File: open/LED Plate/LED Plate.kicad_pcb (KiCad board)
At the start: 2 copper layers, 10 x 13.5 mm, 2 parts, among them J1 Conn_01x02

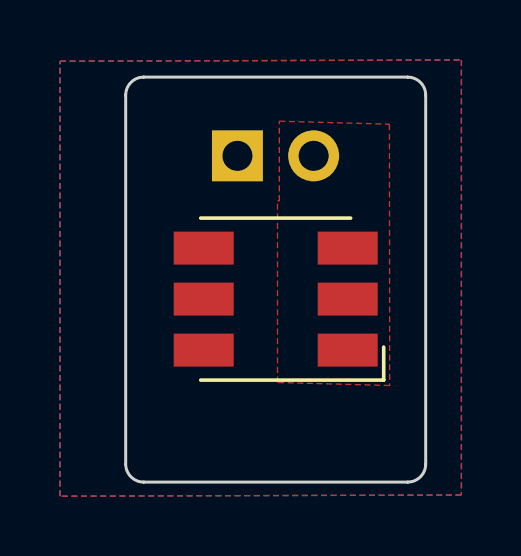
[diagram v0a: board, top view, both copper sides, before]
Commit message: L1-Final Version, L1 Single MUX test
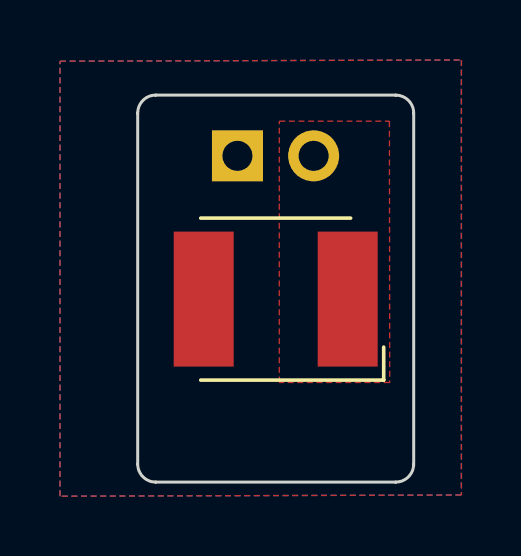
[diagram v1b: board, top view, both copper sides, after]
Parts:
- D1: value LED_RGB -> LED; footprint LED_SMD:LED_RGB_5050-6 -> 2024l1:LED5050
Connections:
- D1 pad 1: +3V3 -> GND
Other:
- board size 10 x 13.5 mm -> 9.2 x 12.9 mm
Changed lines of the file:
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@@
   (net 1 "GND")
   (net 2 "+3V3")
-  (footprint "LED_SMD:LED_RGB_5050-6" (layer "F.Cu")
+  (footprint "2024l1:LED5050" (layer "F.Cu")
     (at 148.5 105.4 180)
-    (descr "http://cdn.sparkfun.com/datasheets/Components/LED/5060BRG4.pdf")
-    (tags "RGB LED 5050-6")
     (property "Sheetfile" "LED Plate.kicad_sch")
     (property "Sheetname" "")
-    (property "ki_description" "RGB LED, 6 pin package")
-    (property "ki_keywords" "LED RGB diode")
+    (property "ki_description" "Light emitting diode")
+    (property "ki_keywords" "LED diode")
     (attr smd)
-    (fp_text reference "D1" (at 0 -3.5) (layer "F.SilkS") hide
-        (effects (font (size 1 1) (thickness 0.15)))
-    )
-    (fp_text value "LED_RGB" (at 0 3.3) (layer "F.Fab")
+    (fp_text reference "D1" (at 0 -0.5 180 unlocked) (layer "F.SilkS") hide
+        (effects (font (size 1 1) (thickness 0.1)))
+    )
+    (fp_text value "LED" (at 0 1 180 unlocked) (layer "F.Fab")
         (effects (font (size 1 1) (thickness 0.15)))
     )
@@
     (fp_circle (center 0 0) (end 0 -1.9)
       (stroke (width 0.1) (type solid)) (fill none) (layer "F.Fab"))
-    (pad "1" smd rect (at -2.4 -1.7 270) (size 1.1 2) (layers "F.Cu" "F.Paste" "F.Mask")
-      (net 2 "+3V3") (pinfunction "RK") (pintype "passive"))
-    (pad "2" smd rect (at -2.4 0 270) (size 1.1 2) (layers "F.Cu" "F.Paste" "F.Mask")
-      (net 2 "+3V3") (pinfunction "GK") (pintype "passive"))
-    (pad "3" smd rect (at -2.4 1.7 270) (size 1.1 2) (layers "F.Cu" "F.Paste" "F.Mask")
-      (net 2 "+3V3") (pinfunction "BK") (pintype "passive"))
-    (pad "4" smd rect (at 2.4 1.7 270) (size 1.1 2) (layers "F.Cu" "F.Paste" "F.Mask")
-      (net 1 "GND") (pinfunction "BA") (pintype "passive"))
-    (pad "5" smd rect (at 2.4 0 270) (size 1.1 2) (layers "F.Cu" "F.Paste" "F.Mask")
-      (net 1 "GND") (pinfunction "GA") (pintype "passive"))
-    (pad "6" smd rect (at 2.4 -1.7 270) (size 1.1 2) (layers "F.Cu" "F.Paste" "F.Mask")
-      (net 1 "GND") (pinfunction "RA") (pintype "passive"))
-    (model "${KICAD6_3DMODEL_DIR}/LED_SMD.3dshapes/LED_RGB_5050-6.wrl"
-      (offset (xyz 0 0 0))
-      (scale (xyz 1 1 1))
-      (rotate (xyz 0 0 0))
-    )
+    (pad "1" smd rect (at 2.4 0 270) (size 4.5 2) (layers "F.Cu" "F.Paste" "F.Mask")
+      (net 1 "GND") (pinfunction "K") (pintype "passive"))
+    (pad "2" smd rect (at -2.4 0 270) (size 4.5 2) (layers "F.Cu" "F.Paste" "F.Mask")
+      (net 2 "+3V3") (pinfunction "A") (pintype "passive"))
   )
   (footprint "Connector_PinHeader_2.54mm:PinHeader_1x02_P2.54mm_Horizontal" (layer "B.Cu")
@@
     )
   )
-  (gr_line (start 144.1 111.5) (end 152.9 111.5)
-    (stroke (width 0.1) (type default)) (layer "Edge.Cuts"))
-  (gr_line (start 143.5 98.6) (end 143.5 110.9)
-    (stroke (width 0.1) (type default)) (layer "Edge.Cuts"))
-  (gr_line (start 153.5 98.6) (end 153.5 110.9)
-    (stroke (width 0.1) (type default)) (layer "Edge.Cuts"))
-  (gr_arc (start 152.9 98) (mid 153.324264 98.175736) (end 153.5 98.6)
-    (stroke (width 0.1) (type default)) (layer "Edge.Cuts"))
-  (gr_arc (start 144.1 111.5) (mid 143.675736 111.324264) (end 143.5 110.9)
-    (stroke (width 0.1) (type default)) (layer "Edge.Cuts"))
-  (gr_arc (start 153.5 110.9) (mid 153.324264 111.324264) (end 152.9 111.5)
-    (stroke (width 0.1) (type default)) (layer "Edge.Cuts"))
-  (gr_arc (start 143.5 98.6) (mid 143.675736 98.175736) (end 144.1 98)
-    (stroke (width 0.1) (type default)) (layer "Edge.Cuts"))
-  (gr_line (start 144.1 98) (end 152.9 98)
-    (stroke (width 0.1) (type default)) (layer "Edge.Cuts"))
+  (gr_line (start 144.5 111.5) (end 152.5 111.5)
+    (stroke (width 0.1) (type default)) (layer "Edge.Cuts"))
+  (gr_arc (start 152.5 98.6) (mid 152.924264 98.775736) (end 153.1 99.2)
+    (stroke (width 0.1) (type default)) (layer "Edge.Cuts"))
+  (gr_arc (start 144.5 111.5) (mid 144.075736 111.324264) (end 143.9 110.9)
+    (stroke (width 0.1) (type default)) (layer "Edge.Cuts"))
+  (gr_arc (start 153.1 110.9) (mid 152.924264 111.324264) (end 152.5 111.5)
+    (stroke (width 0.1) (type default)) (layer "Edge.Cuts"))
+  (gr_line (start 143.9 99.2) (end 143.9 110.9)
+    (stroke (width 0.1) (type default)) (layer "Edge.Cuts"))
+  (gr_arc (start 143.9 99.2) (mid 144.075736 98.775736) (end 144.5 98.6)
+    (stroke (width 0.1) (type default)) (layer "Edge.Cuts"))
+  (gr_line (start 153.1 99.2) (end 153.1 110.9)
+    (stroke (width 0.1) (type default)) (layer "Edge.Cuts"))
+  (gr_line (start 144.5 98.6) (end 152.5 98.6)
+    (stroke (width 0.1) (type default)) (layer "Edge.Cuts"))
+  (dimension (type aligned) (layer "Edge.Cuts")
+    (pts (xy 148.5 98.6) (xy 148.5 111.5))
+    (height -9.15)
+    (gr_text "12.9000 mm" (at 156.5 105.05 90) (layer "Edge.Cuts")
+      (effects (font (size 1 1) (thickness 0.15)))
+    )
+    (format (prefix "") (suffix "") (units 3) (units_format 1) (precision 4))
+    (style (thickness 0.1) (arrow_length 1.27) (text_position_mode 0) (extension_height 0.58642) (extension_offset 0.5) keep_text_aligned)
+  )
+  (dimension (type aligned) (layer "Edge.Cuts")
+    (pts (xy 143.91 104.53) (xy 153.11 104.54))
+    (height 10.358809)
+    (gr_text "9.2000 mm" (at 148.49999 113.743804 359.937722) (layer "Edge.Cuts")
+      (effects (font (size 1 1) (thickness 0.15)))
+    )
+    (format (prefix "") (suffix "") (units 3) (units_format 1) (precision 4))
+    (style (thickness 0.1) (arrow_length 1.27) (text_position_mode 0) (extension_height 0.58642) (extension_offset 0.5) keep_text_aligned)
+  )
   (zone (net 2) (net_name "+3V3") (layer "F.Cu") (hatch edge 0.5)
     (priority 1)
@@
       (pts
         (xy 148.62 99.47)
-        (xy 152.29 99.57)
-        (xy 152.3 108.28)
-        (xy 148.56 108.18)
-        (xy 148.56 102.13)
+        (xy 152.29 99.47)
+        (xy 152.3 108.18)
+        (xy 148.62 108.18)
         (xy 148.62 102.13)
       )
